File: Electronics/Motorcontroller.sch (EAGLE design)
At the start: 59 parts, among them Q1 IRFZ48V, Q2 IRF4905V, Q3 IRFZ48V, Q4 IRF4905V, Q5 IRFZ48V, Q6 IRF4905V, Q7 IRFZ48V, Q8 IRF4905V, T1 BC547, T2 BC547, X3 24V Batt

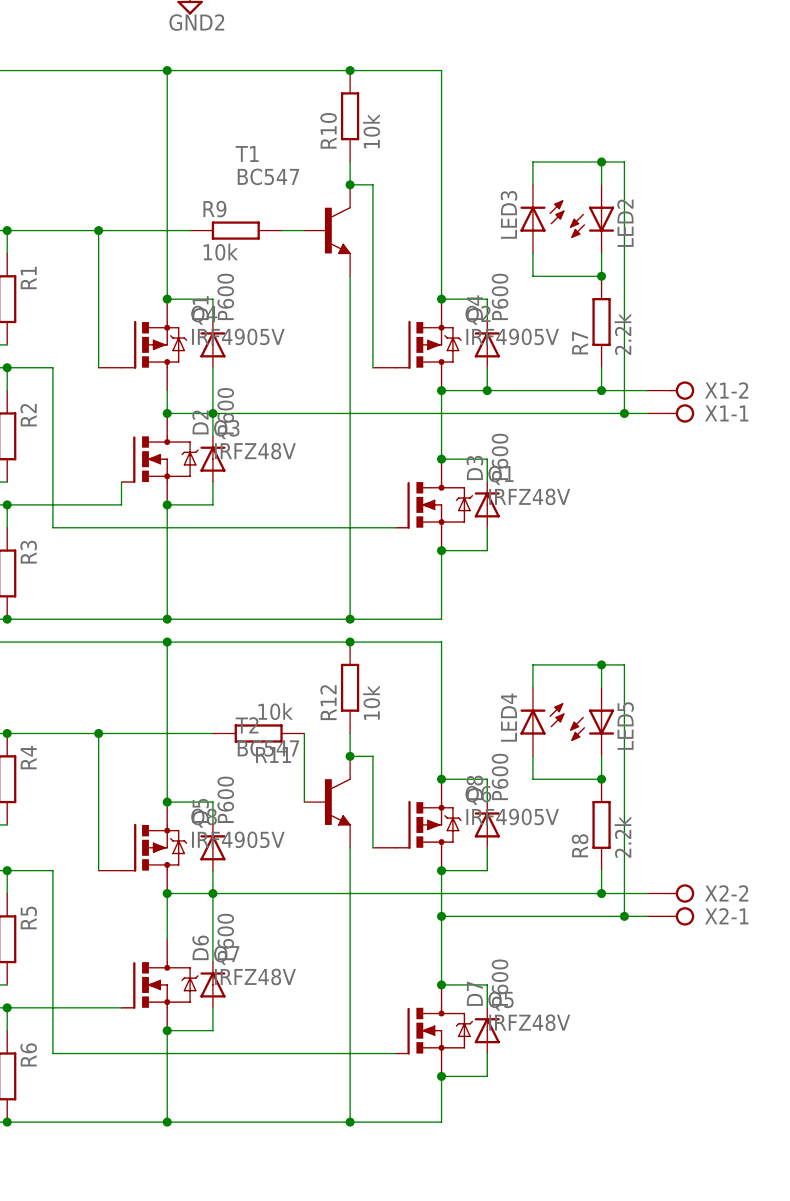
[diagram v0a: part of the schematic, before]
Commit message: Reset to motorcontroller v5.2
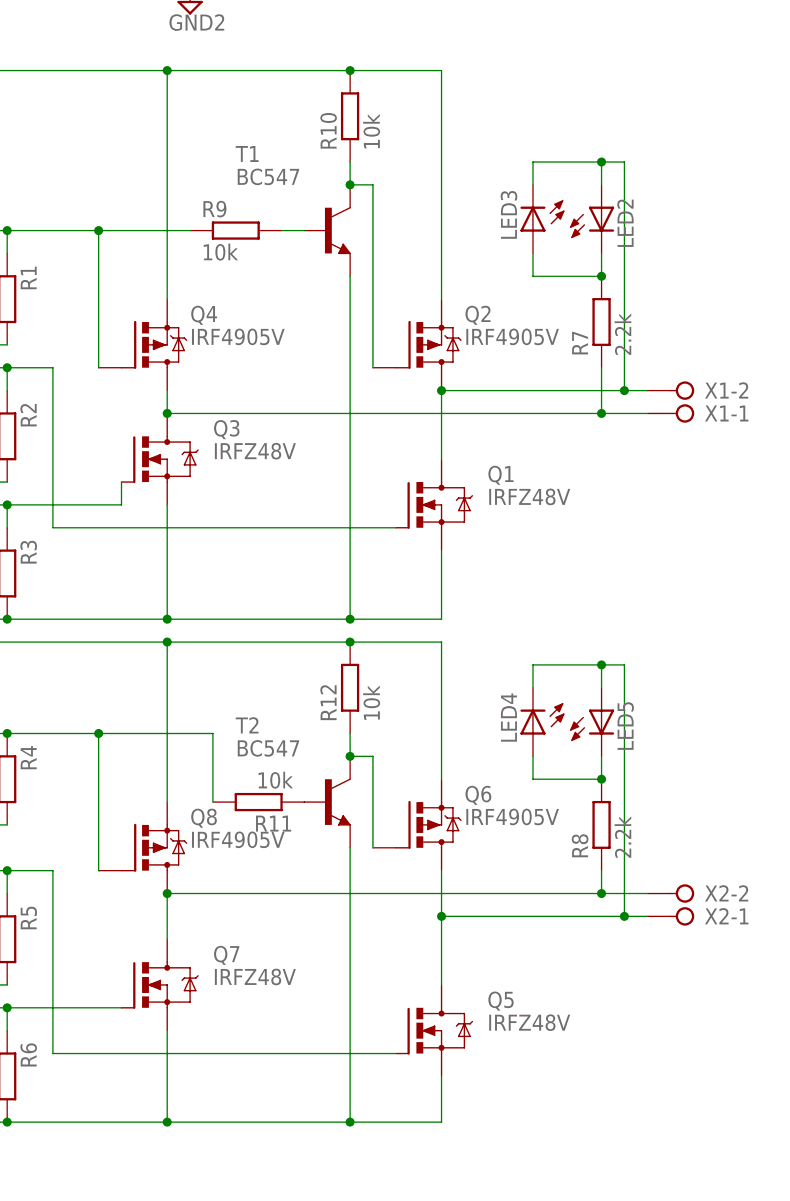
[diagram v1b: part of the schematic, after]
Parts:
- removed D1, D2, D3, D4, D5, D6, D7, D8: P600, diode:P600
- R13: device rcl:R-EU_0207/2V -> rcl:R-EU_0207/10
- R7, R8: device rcl:R-EU_0207/2V -> rcl:R-EU_0207/7
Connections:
- removed net N$36: D1.A, D2.C, LED2.A, LED3.C, Q3.D, Q4.D, X1-1.KL
- removed net N$43: D5.A, D6.C, Q7.D, Q8.D, R8.1, X2-2.KL
- new net N$2: Q3.D, Q4.D, R7.1, X1-1.KL
- new net N$25: Q7.D, Q8.D, R8.1, X2-2.KL
- net +24V: no longer D1.C, D4.C, D5.C, D8.C
- net GND2: no longer D2.A, D3.A, D6.A, D7.A
- net N$1: no longer D7.C, D8.A
- net N$4: now also LED2.A, LED3.C; no longer D3.C, D4.A, R7.1
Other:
- moved on the sheet: R11
